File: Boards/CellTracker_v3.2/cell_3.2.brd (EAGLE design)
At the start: 44.7 x 41.9 mm, 31 parts, among them U2 LMR16020, X1 53261-04

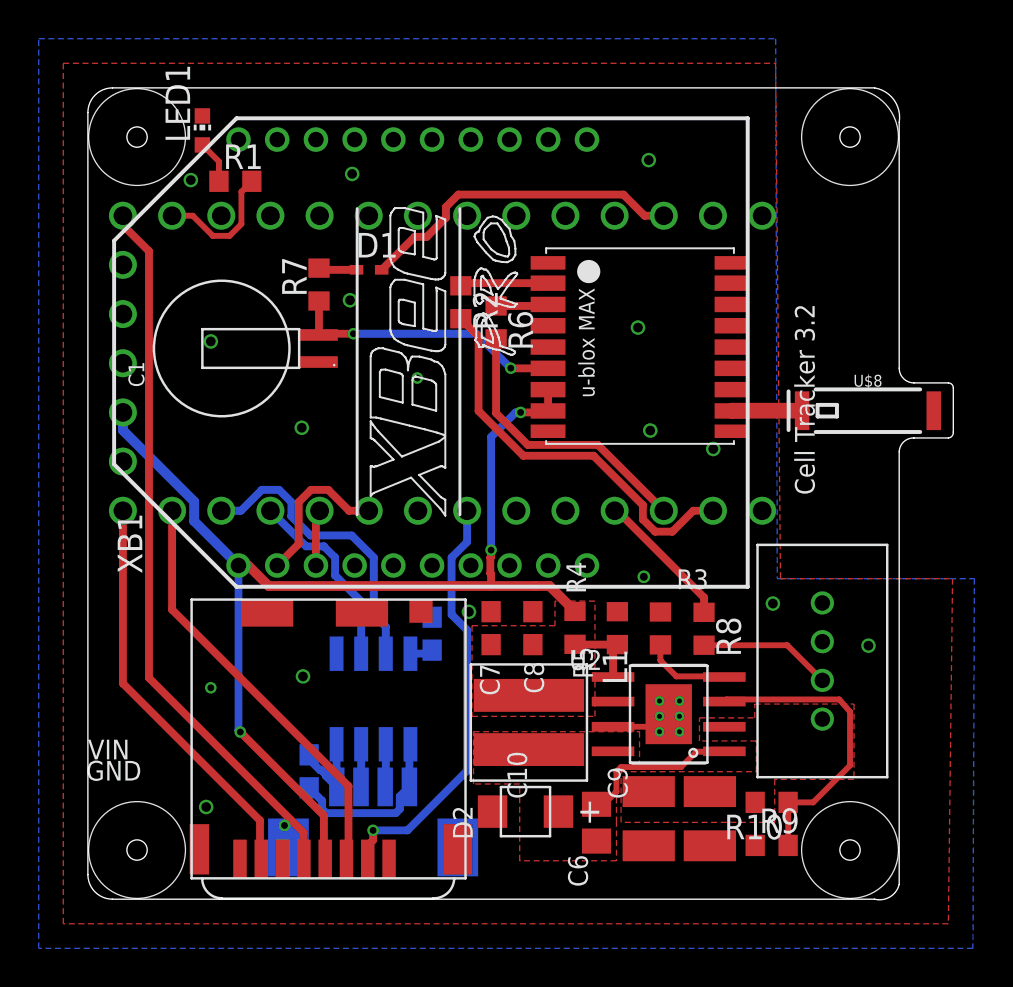
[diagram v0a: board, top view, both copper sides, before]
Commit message: Finishing touches for Cell3.2
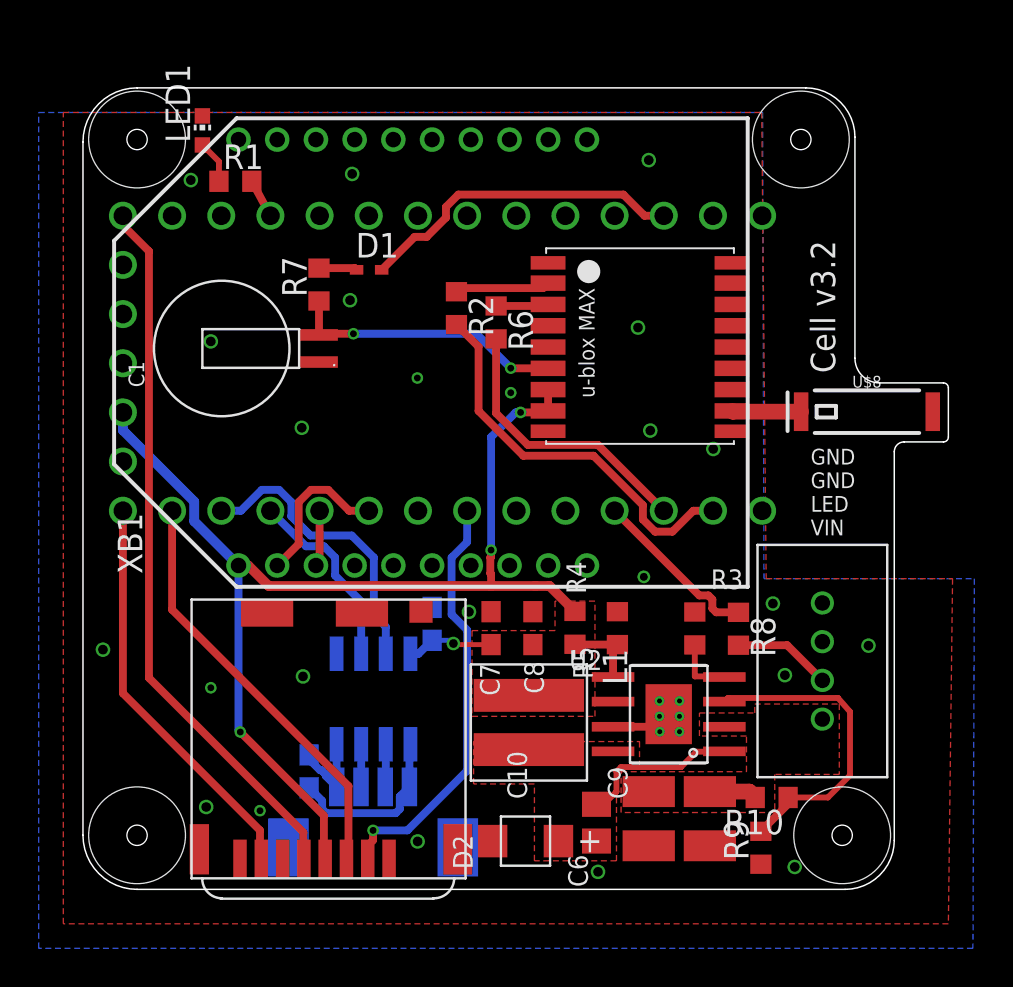
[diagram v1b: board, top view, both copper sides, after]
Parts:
- C1: value (none) -> 0.3F
- moved R3 1.78 mm to (31.4, 14.0)
- moved R8 1.78 mm to (33.6, 14.0)
- moved D2 1.52 mm to (22.6, 3.00)
- moved R9 0.57 mm to (34.8, 2.66), turned to 90 degrees
- moved C3 0.51 mm to (17.8, 14.2)
- moved R2 0.38 mm to (19.0, 30.5)
- moved R10 0.25 mm to (35.3, 5.25)
- moved U$8 0.07 mm to (40.2, 25.2)
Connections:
- removed net N$12: R8.2, U$4.P$1
- removed net VIN: C10.1, C9.1, R10.2, U$1.VIN, U$4.P$2, U2.P$2
- new net IN1: C10.1, C9.1, R10.2, U$4.P$1, U2.P$2
- new net N$11: R8.2, U$4.P$2
- new net NOTUSED: U$1.VIN
- net N$2: now also U$1.16/A2; no longer U$1.14/A0
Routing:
- net N$12: track 6.86 -> 0.00 mm
- net N$11: track 0.00 -> 5.09 mm
- net N$2: track 6.70 -> 2.02 mm
- net +3V3: track 76.4 -> 79.7 mm, vias 3 -> 4
- net IN1: track 0.00 -> 2.47 mm
- net SWITCH_LED: track 7.24 -> 8.84 mm
- net N$8: track 4.46 -> 3.17 mm
- net GND: track 2.50 -> 2.52 mm, vias 24 -> 30
- added copper zone on layer 1, net IN1
- removed copper zone on layer 1, net VIN
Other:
- board size 44.7 x 41.9 mm -> 44.7 x 41.4 mm
- board text added: "3V3>"
- board text added: "</CMD>"
- board text added: "<3V3"
- board text added: "BPP"
- board text added: "Cell v3.2"
- board text added: "GND GND LED VIN"
- board text added: "GND>"
- board text added: "Isolated Conn"
- board text added: "VCC_EX RX_EX TX_EX GND_EX"
- board text added: "VIN: 2S LiPo"
- board text removed: "Cell Tracker 3.2"
- board text removed: "GND"
- board text removed: "VIN"
